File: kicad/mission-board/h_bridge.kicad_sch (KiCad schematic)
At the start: 11 parts, among them J7 H-Bridge Ch A Out, J8 H-Bridge Ch B Out, U13 DRV8833, U14 DRV8833, U3 DRV8833

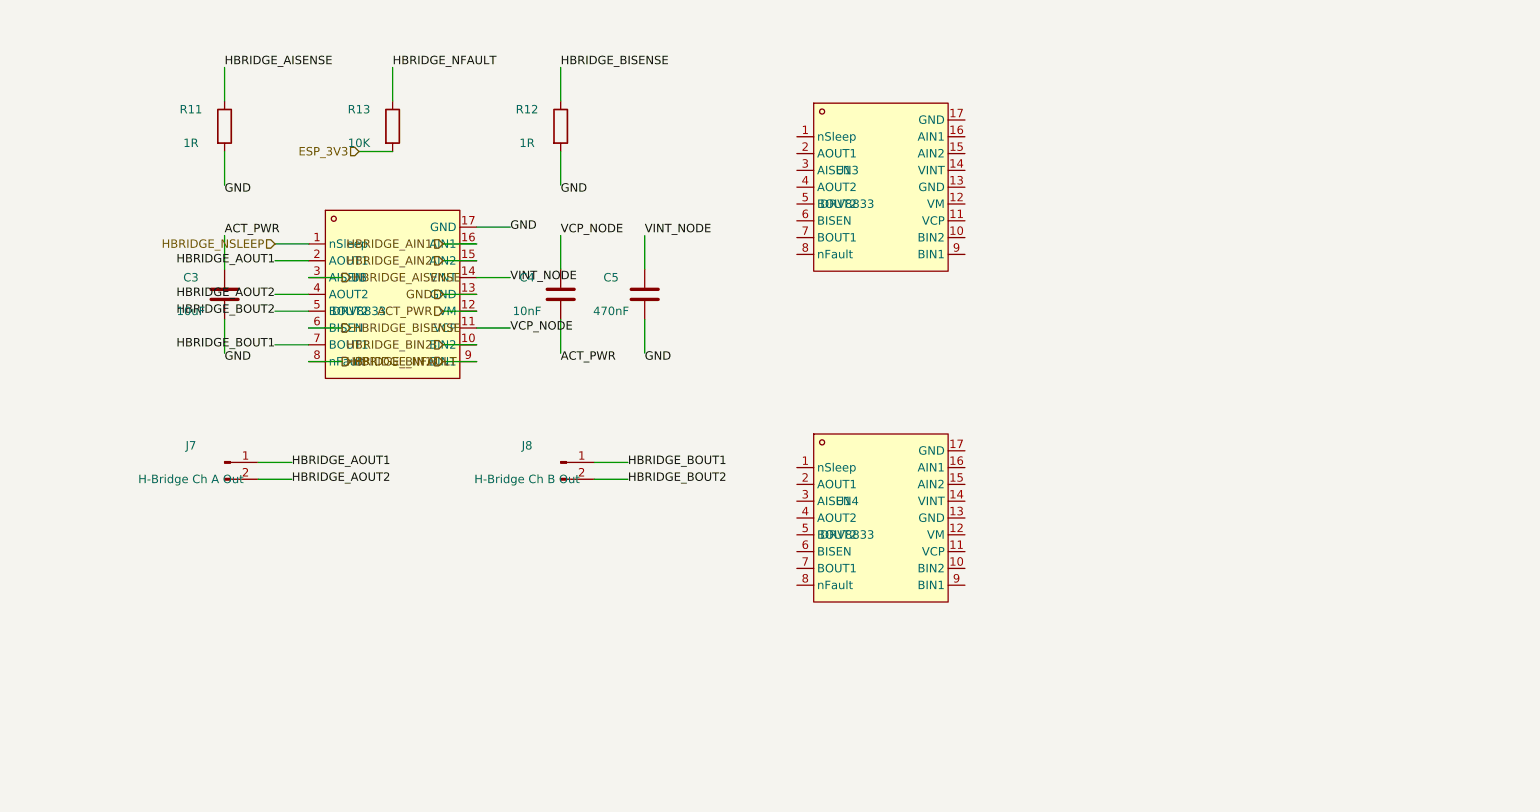
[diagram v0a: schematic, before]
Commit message: pcb progress
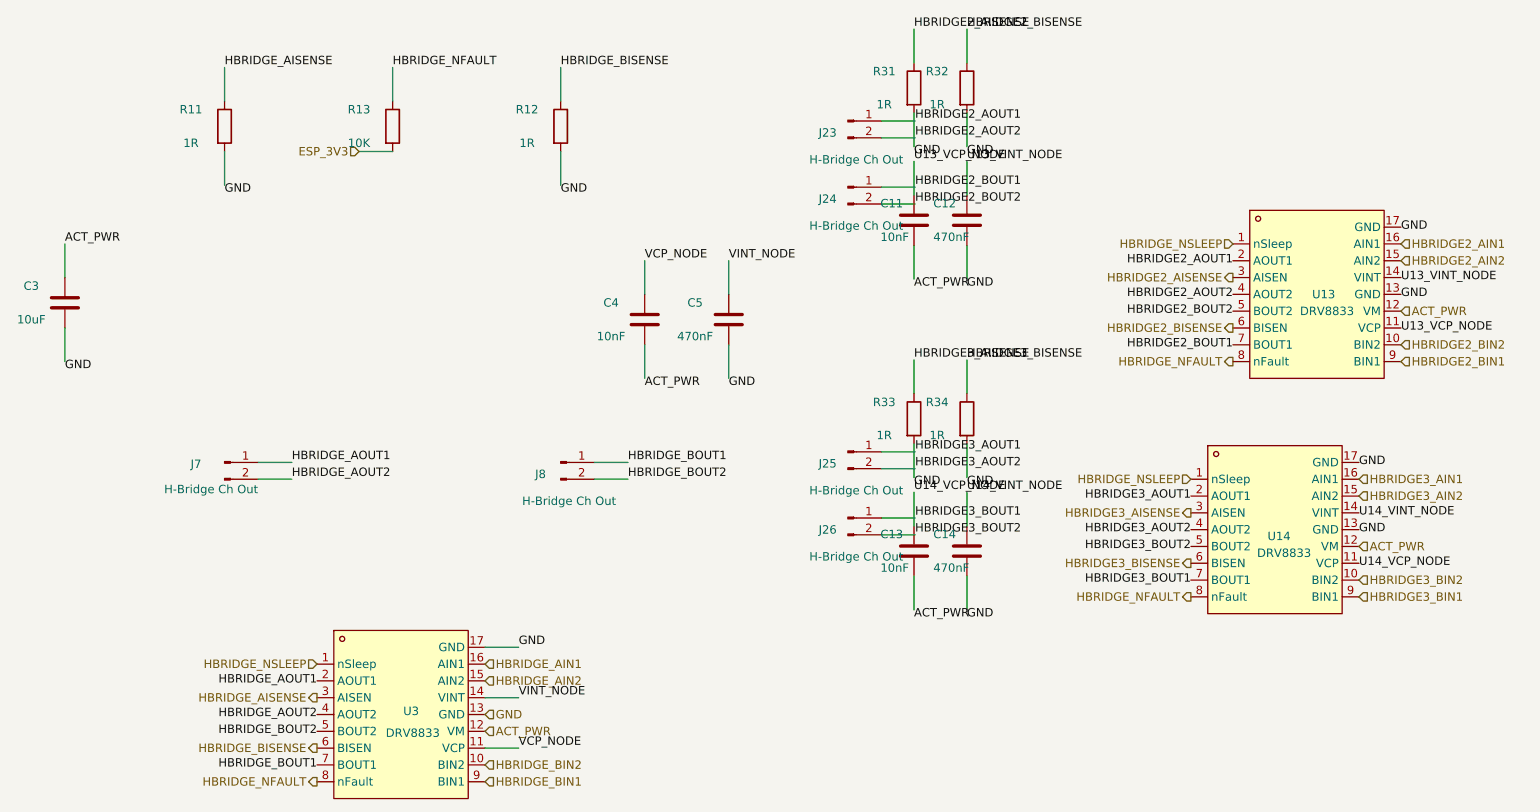
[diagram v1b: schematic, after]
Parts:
- added C11, C13: 10nF, Capacitor_SMD:C_0402_1005Metric, symbol Device:C
- added C12, C14: 470nF, Capacitor_SMD:C_0402_1005Metric, symbol Device:C
- added J23, J24, J25, J26: H-Bridge Ch Out, Connector_JST:JST_XH_B2B-XH-A_1x02_P2.50mm_Vertical, symbol Connector:Conn_01x02_Pin
- added R31, R32, R33, R34: 1R, Resistor_SMD:R_0603_1608Metric, symbol Device:R
- J7: value H-Bridge Ch A Out -> H-Bridge Ch Out
- J8: value H-Bridge Ch B Out -> H-Bridge Ch Out
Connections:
- net ACT_PWR: now also U13.12 (VM), U14.12 (VM), C11.2, C13.2
- net GND: now also U13.13 (GND), U13.17 (GND), U14.13 (GND), U14.17 (GND), C12.2, C14.2, R31.2, R32.2, R33.2, R34.2
- net HBRIDGE_NFAULT: now also U13.8 (nFault), U14.8 (nFault)
- net HBRIDGE_NSLEEP: now also U13.1 (nSleep), U14.1 (nSleep)
- net HBRIDGE3_BIN2: now reaches U14.10 (BIN2)
- net U14_VCP_NODE: now reaches U14.11 (VCP)
- net U14_VCP_NODE: now also C13.1
- net U14_VINT_NODE: now reaches U14.14 (VINT)
- net U14_VINT_NODE: now also C14.1
- net HBRIDGE3_AIN2: now reaches U14.15 (AIN2)
- net HBRIDGE3_AIN1: now reaches U14.16 (AIN1)
- net HBRIDGE3_AOUT1: now reaches U14.2 (AOUT1)
- net HBRIDGE3_AOUT1: now also J25.1 (Pin_1)
- net HBRIDGE3_AISENSE: now reaches U14.3 (AISEN)
- net HBRIDGE3_AISENSE: now also R33.1
- net HBRIDGE3_AOUT2: now reaches U14.4 (AOUT2)
- net HBRIDGE3_AOUT2: now also J25.2 (Pin_2)
- net HBRIDGE3_BOUT2: now reaches U14.5 (BOUT2)
- net HBRIDGE3_BOUT2: now also J26.2 (Pin_2)
- net HBRIDGE3_BISENSE: now reaches U14.6 (BISEN)
- net HBRIDGE3_BISENSE: now also R34.1
- net HBRIDGE3_BOUT1: now reaches U14.7 (BOUT1)
- net HBRIDGE3_BOUT1: now also J26.1 (Pin_1)
- net HBRIDGE3_BIN1: now reaches U14.9 (BIN1)
- net HBRIDGE2_BIN2: now reaches U13.10 (BIN2)
- net U13_VCP_NODE: now reaches U13.11 (VCP)
- net U13_VCP_NODE: now also C11.1
- net U13_VINT_NODE: now reaches U13.14 (VINT)
- net U13_VINT_NODE: now also C12.1
- net HBRIDGE2_AIN2: now reaches U13.15 (AIN2)
- net HBRIDGE2_AIN1: now reaches U13.16 (AIN1)
- net HBRIDGE2_AOUT1: now reaches U13.2 (AOUT1)
- net HBRIDGE2_AOUT1: now also J23.1 (Pin_1)
- net HBRIDGE2_AISENSE: now reaches U13.3 (AISEN)
- net HBRIDGE2_AISENSE: now also R31.1
- net HBRIDGE2_AOUT2: now reaches U13.4 (AOUT2)
- net HBRIDGE2_AOUT2: now also J23.2 (Pin_2)
- net HBRIDGE2_BOUT2: now reaches U13.5 (BOUT2)
- net HBRIDGE2_BOUT2: now also J24.2 (Pin_2)
- net HBRIDGE2_BISENSE: now reaches U13.6 (BISEN)
- net HBRIDGE2_BISENSE: now also R32.1
- net HBRIDGE2_BOUT1: now reaches U13.7 (BOUT1)
- net HBRIDGE2_BOUT1: now also J24.1 (Pin_1)
- net HBRIDGE2_BIN1: now reaches U13.9 (BIN1)
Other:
- moved on the sheet: C3, C4, C5, U13, U14, U3
